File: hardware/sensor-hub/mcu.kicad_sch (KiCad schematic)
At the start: 48 parts, among them J1 Conn_ARM_JTAG_SWD_10, J10 BATT, J2 Micro_SD_Card_Det2, J8 UART_CONN, SW1 SW_Push, U1 STM32F411CEUx, U4 PCAL6408ABS, Y2 32.768kHz, Y3 16MHz

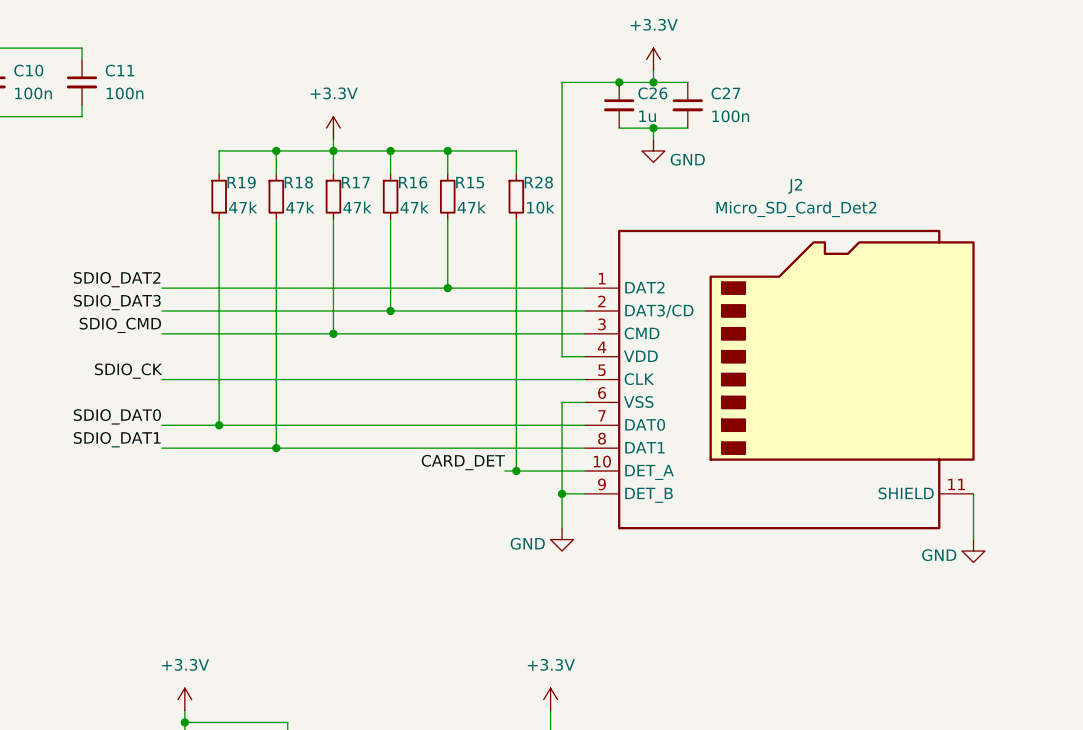
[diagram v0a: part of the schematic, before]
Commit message: Core layout done
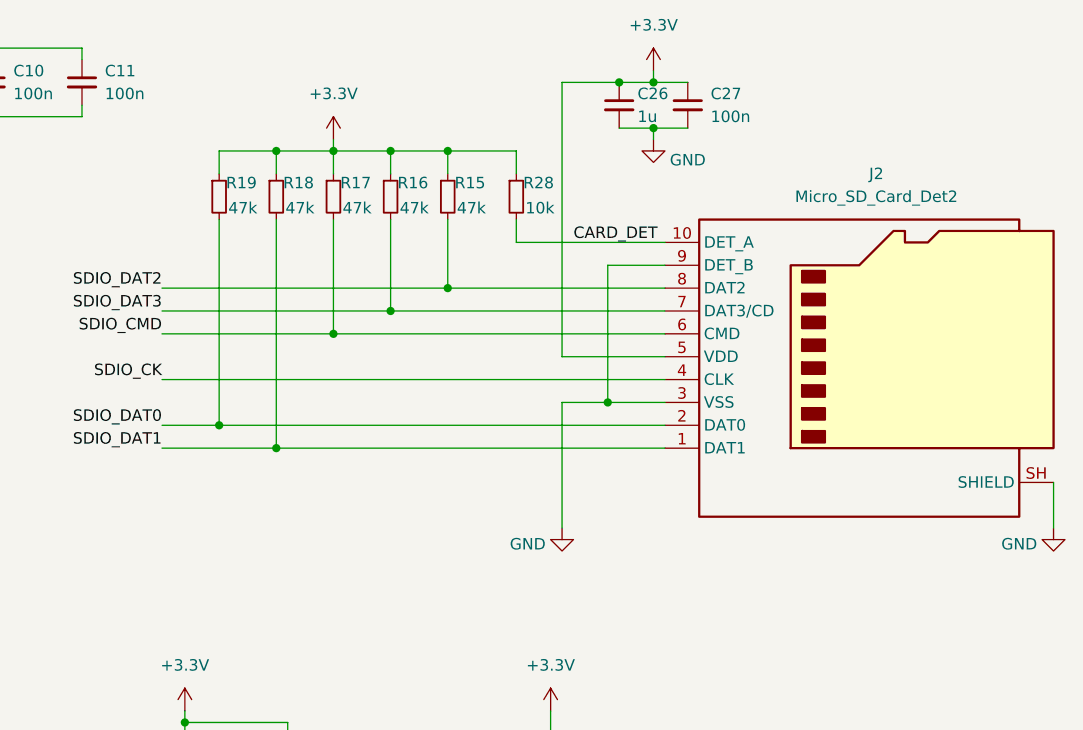
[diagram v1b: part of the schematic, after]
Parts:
- removed J2: Micro_SD_Card_Det2, sensor-hub-footprints:MicroSD_Det2, symbol Connector:Micro_SD_Card_Det2
- added J2: Micro_SD_Card_Det2, sensor-hub-footprints:MicroSD_Det2, symbol sensor-hub-lib:Micro_SD_Card_Det2
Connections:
- net +3.3V: now also J2.5 (VDD)
- net CARD_DET: now also J2.10 (DET_A)
- net GND: now also J2.3 (VSS), J2.9 (DET_B), J2.SH (SHIELD)
- net SDIO_CK: now also J2.4 (CLK)
- net SDIO_CMD: now also J2.6 (CMD)
- net SDIO_DAT0: now also J2.2 (DAT0)
- net SDIO_DAT1: now also J2.1 (DAT1)
- net SDIO_DAT2: now also J2.8 (DAT2)
- net SDIO_DAT3: now also J2.7 (DAT3/CD)
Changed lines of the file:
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@@
 	)
 	(junction
-		(at 218.44 71.12)
+		(at 228.6 63.5)
 		(diameter 0)
 		(color 0 0 0 0)
@@
 	)
 	(junction
-		(at 223.52 73.66)
-		(diameter 0)
-		(color 0 0 0 0)
-	)
-	(junction
 		(at 226.06 101.6)
 		(diameter 0)
@@
 	(wire
 		(pts
-			(xy 226.06 63.5) (xy 223.52 63.5)
+			(xy 223.52 63.5) (xy 228.6 63.5)
 		)
 		(stroke
@@
 	(wire
 		(pts
-			(xy 210.82 50.8) (xy 226.06 50.8)
+			(xy 210.82 50.8) (xy 234.95 50.8)
+		)
+		(stroke
+			(width 0)
+			(type default)
+		)
+	)
+	(wire
+		(pts
+			(xy 228.6 63.5) (xy 234.95 63.5)
 		)
 		(stroke
@@
 	(wire
 		(pts
+			(xy 218.44 45.72) (xy 234.95 45.72)
+		)
+		(stroke
+			(width 0)
+			(type default)
+		)
+	)
+	(wire
+		(pts
 			(xy 156.21 130.81) (xy 156.21 133.35)
 		)
@@
 	(wire
 		(pts
-			(xy 149.86 24.13) (xy 140.97 24.13)
+			(xy 234.95 48.26) (xy 228.6 48.26)
 		)
 		(stroke
@@
 	(wire
 		(pts
-			(xy 218.44 43.18) (xy 218.44 71.12)
+			(xy 149.86 24.13) (xy 140.97 24.13)
 		)
 		(stroke
@@
 	(wire
 		(pts
-			(xy 223.52 73.66) (xy 226.06 73.66)
+			(xy 218.44 43.18) (xy 218.44 45.72)
 		)
 		(stroke
@@
 	(wire
 		(pts
-			(xy 218.44 71.12) (xy 226.06 71.12)
-		)
-		(stroke
-			(width 0)
-			(type default)
-		)
-	)
-	(wire
-		(pts
 			(xy 59.69 73.66) (xy 87.63 73.66)
 		)
@@
 	(wire
 		(pts
-			(xy 269.24 73.66) (xy 269.24 78.74)
-		)
-		(stroke
-			(width 0)
-			(type default)
-		)
-	)
-	(wire
-		(pts
 			(xy 86.36 91.44) (xy 87.63 91.44)
 		)
@@
 	(wire
 		(pts
-			(xy 217.17 71.12) (xy 218.44 71.12)
-		)
-		(stroke
-			(width 0)
-			(type default)
-		)
-	)
-	(wire
-		(pts
 			(xy 123.19 81.28) (xy 137.16 81.28)
 		)
@@
 	(wire
 		(pts
-			(xy 223.52 73.66) (xy 223.52 77.47)
-		)
-		(stroke
-			(width 0)
-			(type default)
-		)
-	)
-	(wire
-		(pts
 			(xy 123.19 50.8) (xy 137.16 50.8)
 		)
@@
 	(wire
 		(pts
-			(xy 223.52 63.5) (xy 223.52 73.66)
+			(xy 223.52 63.5) (xy 223.52 77.47)
 		)
 		(stroke
@@
 	(wire
 		(pts
-			(xy 198.12 55.88) (xy 226.06 55.88)
+			(xy 198.12 55.88) (xy 234.95 55.88)
 		)
 		(stroke
@@
 	(wire
 		(pts
-			(xy 179.07 60.96) (xy 226.06 60.96)
+			(xy 179.07 60.96) (xy 234.95 60.96)
 		)
 		(stroke
@@
 	(wire
 		(pts
+			(xy 278.13 72.39) (xy 278.13 77.47)
+		)
+		(stroke
+			(width 0)
+			(type default)
+		)
+	)
+	(wire
+		(pts
 			(xy 243.84 146.05) (xy 243.84 137.16)
 		)
@@
 	(wire
 		(pts
-			(xy 185.42 66.04) (xy 226.06 66.04)
+			(xy 185.42 66.04) (xy 234.95 66.04)
 		)
 		(stroke
@@
 	(wire
 		(pts
-			(xy 226.06 58.42) (xy 223.52 58.42)
+			(xy 223.52 58.42) (xy 234.95 58.42)
 		)
 		(stroke
@@
 	(wire
 		(pts
-			(xy 204.47 53.34) (xy 226.06 53.34)
+			(xy 204.47 53.34) (xy 234.95 53.34)
 		)
 		(stroke
@@
 	(wire
 		(pts
-			(xy 191.77 68.58) (xy 226.06 68.58)
+			(xy 191.77 68.58) (xy 234.95 68.58)
 		)
 		(stroke
@@
 		)
 	)
+	(wire
+		(pts
+			(xy 228.6 48.26) (xy 228.6 63.5)
+		)
+		(stroke
+			(width 0)
+			(type default)
+		)
+	)
 	(text "BOOT[1:0]:\nx0 - Flash\n01 - Bootloader\n11 - SRAM\n"
 		(exclude_from_sim no)
@@
 	)
 	(label "CARD_DET"
-		(at 217.17 71.12 180)
+		(at 224.79 45.72 0)
 		(effects
 			(font
 				(size 1.27 1.27)
 			)
-			(justify right bottom)
+			(justify left bottom)
 		)
 	)
@@
 	(symbol
 		(lib_id "power:GND")
-		(at 269.24 78.74 0)
+		(at 278.13 77.47 0)
 		(unit 1)
 		(exclude_from_sim no)
@@
 		(dnp no)
 		(property "Reference" "#PWR51"
-			(at 269.24 85.09 0)
+			(at 278.13 83.82 0)
 			(effects
 				(font
@@
 		)
 		(property "Value" "GND"
-			(at 265.43 80.518 0)
+			(at 274.32 79.248 0)
 			(effects
 				(font
@@
 		)
 		(property "Footprint" ""
-			(at 269.24 78.74 0)
+			(at 278.13 77.47 0)
 			(effects
 				(font
@@
 		)
 		(property "Datasheet" ""
-			(at 269.24 78.74 0)
+			(at 278.13 77.47 0)
 			(effects
 				(font
@@
 		)
 		(property "Description" "Power symbol creates a global label with name \"GND\" , ground"
-			(at 269.24 78.74 0)
+			(at 278.13 77.47 0)
 			(effects
 				(font
@@
 	)
 	(symbol
-		(lib_id "Connector:Micro_SD_Card_Det2")
-		(at 248.92 60.96 0)
-		(unit 1)
-		(exclude_from_sim no)
-		(in_bom yes)
-		(on_board yes)
-		(dnp no)
-		(fields_autoplaced yes)
-		(property "Reference" "J2"
-			(at 249.555 39.37 0)
-			(effects
-				(font
-					(size 1.27 1.27)
-				)
-			)
-		)
-		(property "Value" "Micro_SD_Card_Det2"
-			(at 249.555 41.91 0)
-			(effects
-				(font
-					(size 1.27 1.27)
-				)
-			)
-		)
-		(property "Footprint" "sensor-hub-footprints:MicroSD_Det2"
-			(at 300.99 43.18 0)
-			(effects
-				(font
-					(size 1.27 1.27)
-				)
-				(hide yes)
-			)
-		)
-		(property "Datasheet" "https://www.hirose.com/en/product/document?clcode=&productname=&series=DM3&documenttype=Catalog&lang=en&documentid=D49662_en"
-			(at 251.46 58.42 0)
-			(effects
-				(font
-					(size 1.27 1.27)
-				)
-				(hide yes)
-			)
-		)
-		(property "Description" "Micro SD Card Socket with two card detection pins"
-			(at 248.92 60.96 0)
-			(effects
-				(font
-					(size 1.27 1.27)
-				)
-				(hide yes)
-			)
-		)
-		(pin "5"
-		)
-		(pin "7"
-		)
-		(pin "10"
-		)
-		(pin "1"
-		)
-		(pin "8"
-		)
-		(pin "9"
-		)
-		(pin "4"
-		)
-		(pin "11"
-		)
-		(pin "3"
-		)
-		(pin "2"
-		)
-		(pin "6"
-		)
-		(instances
-			(project ""
-				(path "/e168ef7b-16e4-493f-b63c-2f69374fc890/acb07f68-122e-4e37-938b-04e6ced67923"
-					(reference "J2")
-					(unit 1)
-				)
-			)
-		)
-	)
-	(symbol
 		(lib_id "power:GND")
 		(at 35.56 39.37 0)
@@
 					(unit 1)
 				)
+			)
+		)
+	)
+	(symbol
+		(lib_id "sensor-hub-lib:Micro_SD_Card_Det2")
+		(at 257.81 59.69 0)
+		(unit 1)
+		(exclude_from_sim no)
+		(in_bom yes)
+		(on_board yes)
+		(dnp no)
+		(fields_autoplaced yes)
+		(property "Reference" "J2"
+			(at 258.445 38.1 0)
+			(effects
+				(font
+					(size 1.27 1.27)
+				)
+			)
+		)
+		(property "Value" "Micro_SD_Card_Det2"
+			(at 258.445 40.64 0)
+			(effects
+				(font
+					(size 1.27 1.27)
+				)
+			)
+		)
+		(property "Footprint" "sensor-hub-footprints:MicroSD_Det2"
+			(at 309.88 41.91 0)
+			(effects
+				(font
+					(size 1.27 1.27)
+				)
+				(hide yes)
+			)
+		)
+		(property "Datasheet" ""
+			(at 260.35 57.15 0)
+			(effects
+				(font
+					(size 1.27 1.27)
+				)
+				(hide yes)
+			)
+		)
+		(property "Description" "Micro SD Card Socket with two card detection pins"
+			(at 257.81 59.69 0)
+			(effects
+				(font
+					(size 1.27 1.27)
+				)
+				(hide yes)
+			)
+		)
+		(pin "1"
+		)
+		(pin "5"
+		)
+		(pin "8"
+		)
+		(pin "10"
+		)
+		(pin "2"
+		)
+		(pin "6"
+		)
+		(pin "7"
+		)
+		(pin "4"
+		)
+		(pin "3"
+		)
+		(pin "9"
+		)
+		(pin "SH"
+		)
+		(instances
+			(project ""
+				(path "/e168ef7b-16e4-493f-b63c-2f69374fc890/acb07f68-122e-4e37-938b-04e6ced67923"
+					(reference "J2")
+					(unit 1)
+				)

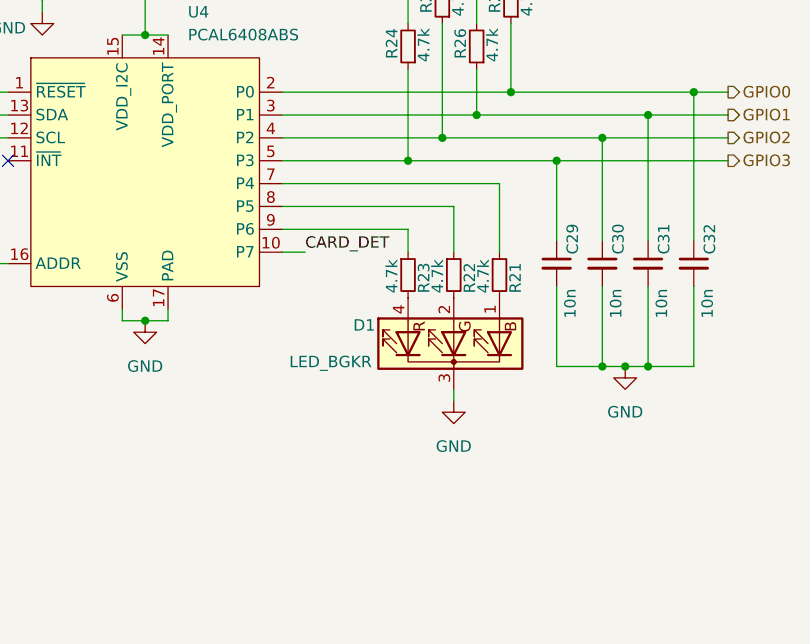
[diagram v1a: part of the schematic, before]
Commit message: Most layout done
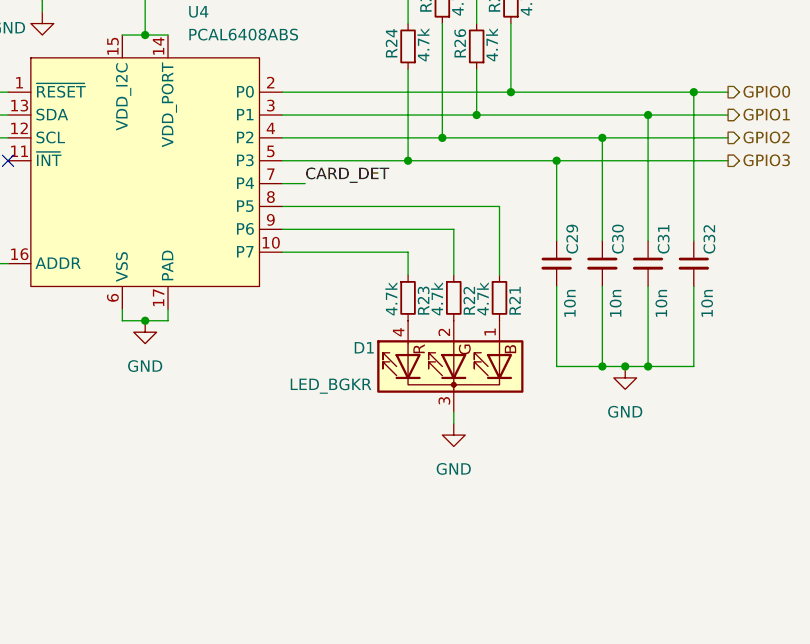
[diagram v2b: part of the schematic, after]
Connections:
- net CARD_DET: now also U4.7 (P4); no longer U4.10 (P7)
- net at R21.1: now also U4.8 (P5); no longer U4.7 (P4)
- net at R22.1: now also U4.9 (P6); no longer U4.8 (P5)
- net at R23.1: now also U4.10 (P7); no longer U4.9 (P6)
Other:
- moved on the sheet: D1, R21, R22, R23
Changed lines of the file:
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@@
 	(wire
 		(pts
+			(xy 208.28 125.73) (xy 210.82 125.73)
+		)
+		(stroke
+			(width 0)
+			(type default)
+		)
+	)
+	(wire
+		(pts
 			(xy 248.92 118.11) (xy 248.92 132.08)
 		)
@@
 	(wire
 		(pts
-			(xy 227.33 148.59) (xy 227.33 149.86)
+			(xy 227.33 151.13) (xy 227.33 152.4)
 		)
 		(stroke
@@
 	(wire
 		(pts
-			(xy 208.28 125.73) (xy 232.41 125.73)
+			(xy 208.28 128.27) (xy 232.41 128.27)
 		)
 		(stroke
@@
 	(wire
 		(pts
-			(xy 208.28 133.35) (xy 210.82 133.35)
-		)
-		(stroke
-			(width 0)
-			(type default)
-		)
-	)
-	(wire
-		(pts
-			(xy 227.33 128.27) (xy 227.33 133.35)
+			(xy 227.33 130.81) (xy 227.33 135.89)
 		)
 		(stroke
@@
 	(wire
 		(pts
-			(xy 208.28 128.27) (xy 227.33 128.27)
+			(xy 208.28 130.81) (xy 227.33 130.81)
 		)
 		(stroke
@@
 	(wire
 		(pts
-			(xy 232.41 125.73) (xy 232.41 133.35)
+			(xy 232.41 128.27) (xy 232.41 135.89)
 		)
 		(stroke
@@
 	(wire
 		(pts
-			(xy 222.25 133.35) (xy 222.25 130.81)
+			(xy 222.25 135.89) (xy 222.25 133.35)
 		)
 		(stroke
@@
 	(wire
 		(pts
-			(xy 222.25 130.81) (xy 208.28 130.81)
+			(xy 222.25 133.35) (xy 208.28 133.35)
 		)
 		(stroke
@@
 	)
 	(label "CARD_DET"
-		(at 210.82 133.35 0)
+		(at 210.82 125.73 0)
 		(effects
 			(font
@@
 	(symbol
 		(lib_id "Device:R_Small")
-		(at 227.33 135.89 0)
+		(at 227.33 138.43 0)
 		(unit 1)
 		(exclude_from_sim no)
@@
 		(dnp no)
 		(property "Reference" "R22"
-			(at 229.108 137.922 90)
+			(at 229.108 140.462 90)
 			(effects
 				(font
@@
 		)
 		(property "Value" "4.7k"
-			(at 225.552 137.922 90)
+			(at 225.552 140.462 90)
 			(effects
 				(font
@@
 		)
 		(property "Footprint" "Resistor_SMD:R_0603_1608Metric"
-			(at 227.33 135.89 0)
+			(at 227.33 138.43 0)
 			(effects
 				(font
@@
 		)
 		(property "Datasheet" "~"
-			(at 227.33 135.89 0)
+			(at 227.33 138.43 0)
 			(effects
 				(font
@@
 		)
 		(property "Description" "Resistor, small symbol"
-			(at 227.33 135.89 0)
+			(at 227.33 138.43 0)
 			(effects
 				(font
@@
 	(symbol
 		(lib_id "power:GND")
-		(at 227.33 149.86 0)
+		(at 227.33 152.4 0)
 		(unit 1)
 		(exclude_from_sim no)
@@
 		(fields_autoplaced yes)
 		(property "Reference" "#PWR54"
-			(at 227.33 156.21 0)
+			(at 227.33 158.75 0)
 			(effects
 				(font
@@
 		)
 		(property "Value" "GND"
-			(at 227.33 154.94 0)
+			(at 227.33 157.48 0)
 			(effects
 				(font
@@
 		)
 		(property "Footprint" ""
-			(at 227.33 149.86 0)
+			(at 227.33 152.4 0)
 			(effects
 				(font
@@
 		)
 		(property "Datasheet" ""
-			(at 227.33 149.86 0)
+			(at 227.33 152.4 0)
 			(effects
 				(font
@@
 		)
 		(property "Description" "Power symbol creates a global label with name \"GND\" , ground"
-			(at 227.33 149.86 0)
+			(at 227.33 152.4 0)
 			(effects
 				(font
@@
 	(symbol
 		(lib_id "Device:R_Small")
-		(at 222.25 135.89 0)
+		(at 222.25 138.43 0)
 		(unit 1)
 		(exclude_from_sim no)
@@
 		(dnp no)
 		(property "Reference" "R23"
-			(at 224.028 137.922 90)
+			(at 224.028 140.462 90)
 			(effects
 				(font
@@
 		)
 		(property "Value" "4.7k"
-			(at 220.472 137.922 90)
+			(at 220.472 140.462 90)
 			(effects
 				(font
@@
 		)
 		(property "Footprint" "Resistor_SMD:R_0603_1608Metric"
-			(at 222.25 135.89 0)
+			(at 222.25 138.43 0)
 			(effects
 				(font
@@
 		)
 		(property "Datasheet" "~"
-			(at 222.25 135.89 0)
+			(at 222.25 138.43 0)
 			(effects
 				(font
@@
 		)
 		(property "Description" "Resistor, small symbol"
-			(at 222.25 135.89 0)
+			(at 222.25 138.43 0)
 			(effects
 				(font
@@
 	(symbol
 		(lib_id "Device:LED_BGKR")
-		(at 227.33 143.51 90)
+		(at 227.33 146.05 90)
 		(unit 1)
 		(exclude_from_sim no)
@@
 		(dnp no)
 		(property "Reference" "D1"
-			(at 216.154 141.478 90)
+			(at 216.154 144.018 90)
 			(effects
 				(font
@@
 		)
 		(property "Value" "LED_BGKR"
-			(at 209.042 145.542 90)
+			(at 209.042 148.082 90)
 			(effects
 				(font
@@
 		)
 		(property "Footprint" "LED_SMD:LED_Cree-PLCC4_3.2x2.8mm_CCW"
-			(at 228.6 143.51 0)
+			(at 228.6 146.05 0)
 			(effects
 				(font
@@
 		)
 		(property "Datasheet" "~"
-			(at 228.6 143.51 0)
+			(at 228.6 146.05 0)
 			(effects
 				(font
@@
 		)
 		(property "Description" "RGB LED, blue/green/cathode/red"
-			(at 227.33 143.51 0)
+			(at 227.33 146.05 0)
 			(effects
 				(font
@@
 	(symbol
 		(lib_id "Device:R_Small")
-		(at 232.41 135.89 0)
+		(at 232.41 138.43 0)
 		(unit 1)
 		(exclude_from_sim no)
@@
 		(dnp no)
 		(property "Reference" "R21"
-			(at 234.188 137.922 90)
+			(at 234.188 140.462 90)
 			(effects
 				(font
@@
 		)
 		(property "Value" "4.7k"
-			(at 230.632 137.922 90)
+			(at 230.632 140.462 90)
 			(effects
 				(font
@@
 		)
 		(property "Footprint" "Resistor_SMD:R_0603_1608Metric"
-			(at 232.41 135.89 0)
+			(at 232.41 138.43 0)
 			(effects
 				(font
@@
 		)
 		(property "Datasheet" "~"
-			(at 232.41 135.89 0)
+			(at 232.41 138.43 0)
 			(effects
 				(font
@@
 		)
 		(property "Description" "Resistor, small symbol"
-			(at 232.41 135.89 0)
+			(at 232.41 138.43 0)
 			(effects
 				(font
